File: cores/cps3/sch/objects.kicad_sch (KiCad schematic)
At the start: 0 parts

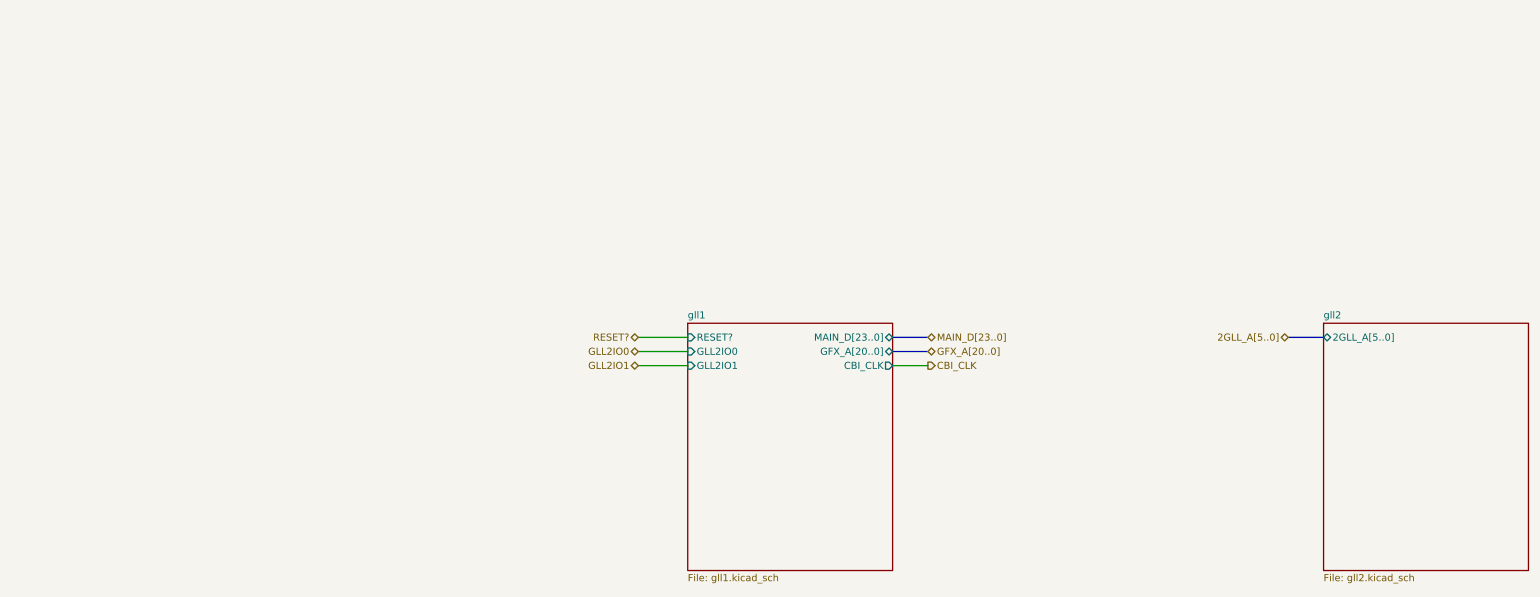
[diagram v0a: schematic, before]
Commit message: update7
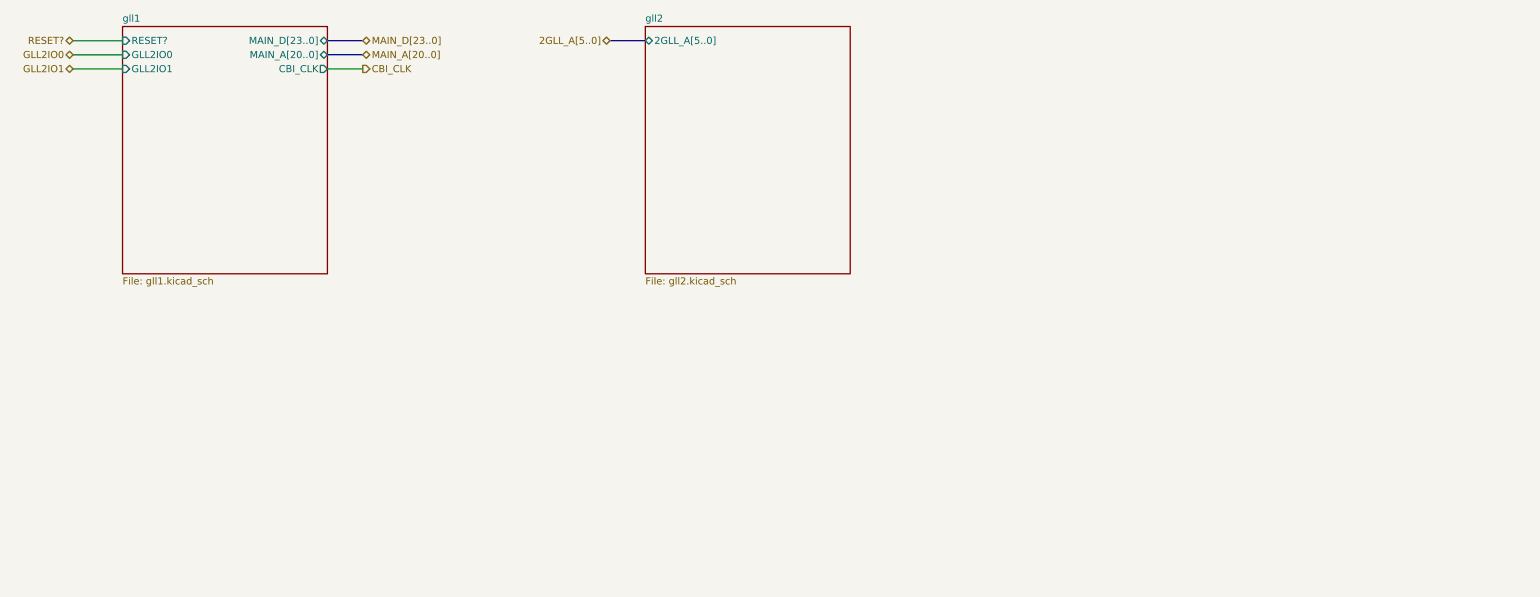
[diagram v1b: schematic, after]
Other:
- sheet gll1 ports: added MAIN_A[20..0]; removed GFX_A[20..0]
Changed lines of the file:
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@@
 (kicad_sch (version 20211123) (generator eeschema)
-  (paper "A3")
+  (paper "A5")
   (title_block
     (title "CP SYSTEM III")
@@
     (comment 1 "E.Triana")
   )
-  (wire (pts (xy 130.81 91.44) (xy 139.7 91.44))
-    (stroke (width 0) (type default) (color 0 0 0 0))
-  )
-  (wire (pts (xy 130.81 96.52) (xy 139.7 96.52))
-    (stroke (width 0) (type default) (color 0 0 0 0))
-  )
-  (bus (pts (xy 176.53 93.98) (xy 182.88 93.98))
-    (stroke (width 0) (type default) (color 0 0 0 0))
-  )
-  (bus (pts (xy 176.53 91.44) (xy 182.88 91.44))
-    (stroke (width 0) (type default) (color 0 0 0 0))
-  )
-  (bus (pts (xy 247.65 91.44) (xy 254 91.44))
-    (stroke (width 0) (type default) (color 0 0 0 0))
-  )
-  (wire (pts (xy 176.53 96.52) (xy 182.88 96.52))
-    (stroke (width 0) (type default) (color 0 0 0 0))
-  )
-  (wire (pts (xy 130.81 93.98) (xy 139.7 93.98))
-    (stroke (width 0) (type default) (color 0 0 0 0))
-  )
-  (image (at 398.78 261.62) (scale 0.294008)
+  (wire (pts (xy 29.21 38.1) (xy 38.1 38.1))
+    (stroke (width 0) (type default) (color 0 0 0 0))
+  )
+  (wire (pts (xy 29.21 43.18) (xy 38.1 43.18))
+    (stroke (width 0) (type default) (color 0 0 0 0))
+  )
+  (bus (pts (xy 74.93 40.64) (xy 81.28 40.64))
+    (stroke (width 0) (type default) (color 0 0 0 0))
+  )
+  (bus (pts (xy 74.93 38.1) (xy 81.28 38.1))
+    (stroke (width 0) (type default) (color 0 0 0 0))
+  )
+  (bus (pts (xy 125.73 38.1) (xy 132.08 38.1))
+    (stroke (width 0) (type default) (color 0 0 0 0))
+  )
+  (wire (pts (xy 74.93 43.18) (xy 81.28 43.18))
+    (stroke (width 0) (type default) (color 0 0 0 0))
+  )
+  (wire (pts (xy 29.21 40.64) (xy 38.1 40.64))
+    (stroke (width 0) (type default) (color 0 0 0 0))
+  )
+  (image (at 186.69 111.76) (scale 0.294008)
     (data
       iVBORw0KGgoAAAANSUhEUgAAAtEAAAGsCAMAAAAsQwu3AAAAA3NCSVQICAjb4U/gAAADAFBMVEX/
@@
     )
   )
-  (hierarchical_label "MAIN_D[23..0]" (shape bidirectional) (at 182.88 91.44 0)
+  (hierarchical_label "MAIN_D[23..0]" (shape bidirectional) (at 81.28 38.1 0)
     (effects (font (size 1.27 1.27)) (justify left))
   )
-  (hierarchical_label "2GLL_A[5..0]" (shape bidirectional) (at 247.65 91.44 180)
-    (effects (font (size 1.27 1.27)) (justify right))
-  )
-  (hierarchical_label "RESET?" (shape tri_state) (at 130.81 91.44 180)
-    (effects (font (size 1.27 1.27)) (justify right))
-  )
-  (hierarchical_label "GLL2IO1" (shape bidirectional) (at 130.81 96.52 180)
-    (effects (font (size 1.27 1.27)) (justify right))
-  )
-  (hierarchical_label "GFX_A[20..0]" (shape tri_state) (at 182.88 93.98 0)
+  (hierarchical_label "2GLL_A[5..0]" (shape bidirectional) (at 125.73 38.1 180)
+    (effects (font (size 1.27 1.27)) (justify right))
+  )
+  (hierarchical_label "RESET?" (shape tri_state) (at 29.21 38.1 180)
+    (effects (font (size 1.27 1.27)) (justify right))
+  )
+  (hierarchical_label "GLL2IO1" (shape bidirectional) (at 29.21 43.18 180)
+    (effects (font (size 1.27 1.27)) (justify right))
+  )
+  (hierarchical_label "MAIN_A[20..0]" (shape tri_state) (at 81.28 40.64 0)
     (effects (font (size 1.27 1.27)) (justify left))
   )
-  (hierarchical_label "CBI_CLK" (shape output) (at 182.88 96.52 0)
+  (hierarchical_label "CBI_CLK" (shape output) (at 81.28 43.18 0)
     (effects (font (size 1.27 1.27)) (justify left))
   )
-  (hierarchical_label "GLL2IO0" (shape tri_state) (at 130.81 93.98 180)
-    (effects (font (size 1.27 1.27)) (justify right))
-  )
-  (sheet (at 254 88.9) (size 36.83 44.45) (fields_autoplaced)
+  (hierarchical_label "GLL2IO0" (shape tri_state) (at 29.21 40.64 180)
+    (effects (font (size 1.27 1.27)) (justify right))
+  )
+  (sheet (at 132.08 35.56) (size 36.83 44.45) (fields_autoplaced)
     (stroke (width 0.1524) (type solid) (color 0 0 0 0))
     (fill (color 0 0 0 0.0000))
-    (property "Sheet name" "gll2" (id 0) (at 254 88.1884 0)
+    (property "Sheet name" "gll2" (id 0) (at 132.08 34.8484 0)
       (effects (font (size 1.27 1.27)) (justify left bottom))
     )
-    (property "Sheet file" "gll2.kicad_sch" (id 1) (at 254 133.9346 0)
+    (property "Sheet file" "gll2.kicad_sch" (id 1) (at 132.08 80.5946 0)
       (effects (font (size 1.27 1.27)) (justify left top))
     )
-    (pin "2GLL_A[5..0]" bidirectional (at 254 91.44 180)
-      (effects (font (size 1.27 1.27)) (justify left))
-    )
-  )
-  (sheet (at 139.7 88.9) (size 36.83 44.45) (fields_autoplaced)
+    (pin "2GLL_A[5..0]" bidirectional (at 132.08 38.1 180)
+      (effects (font (size 1.27 1.27)) (justify left))
+    )
+  )
+  (sheet (at 38.1 35.56) (size 36.83 44.45) (fields_autoplaced)
     (stroke (width 0.1524) (type solid) (color 0 0 0 0))
     (fill (color 0 0 0 0.0000))
-    (property "Sheet name" "gll1" (id 0) (at 139.7 88.1884 0)
+    (property "Sheet name" "gll1" (id 0) (at 38.1 34.8484 0)
       (effects (font (size 1.27 1.27)) (justify left bottom))
     )
-    (property "Sheet file" "gll1.kicad_sch" (id 1) (at 139.7 133.9346 0)
+    (property "Sheet file" "gll1.kicad_sch" (id 1) (at 38.1 80.5946 0)
       (effects (font (size 1.27 1.27)) (justify left top))
     )
-    (pin "CBI_CLK" output (at 176.53 96.52 0)
+    (pin "CBI_CLK" output (at 74.93 43.18 0)
       (effects (font (size 1.27 1.27)) (justify right))
     )
-    (pin "MAIN_D[23..0]" bidirectional (at 176.53 91.44 0)
+    (pin "MAIN_D[23..0]" bidirectional (at 74.93 38.1 0)
       (effects (font (size 1.27 1.27)) (justify right))
     )
-    (pin "GFX_A[20..0]" bidirectional (at 176.53 93.98 0)
+    (pin "RESET?" input (at 38.1 38.1 180)
+      (effects (font (size 1.27 1.27)) (justify left))
+    )
+    (pin "GLL2IO0" input (at 38.1 40.64 180)
+      (effects (font (size 1.27 1.27)) (justify left))
+    )
+    (pin "GLL2IO1" input (at 38.1 43.18 180)
+      (effects (font (size 1.27 1.27)) (justify left))
+    )
+    (pin "MAIN_A[20..0]" bidirectional (at 74.93 40.64 0)
       (effects (font (size 1.27 1.27)) (justify right))
     )
-    (pin "RESET?" input (at 139.7 91.44 180)
-      (effects (font (size 1.27 1.27)) (justify left))
-    )
-    (pin "GLL2IO0" input (at 139.7 93.98 180)
-      (effects (font (size 1.27 1.27)) (justify left))
-    )
-    (pin "GLL2IO1" input (at 139.7 96.52 180)
-      (effects (font (size 1.27 1.27)) (justify left))
-    )
-  )
+  )
